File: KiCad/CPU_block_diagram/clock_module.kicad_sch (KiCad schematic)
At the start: 17 parts, among them SW1 SW_Push, U1 LM555xN, U2 LM555xN, U3 LM555xN

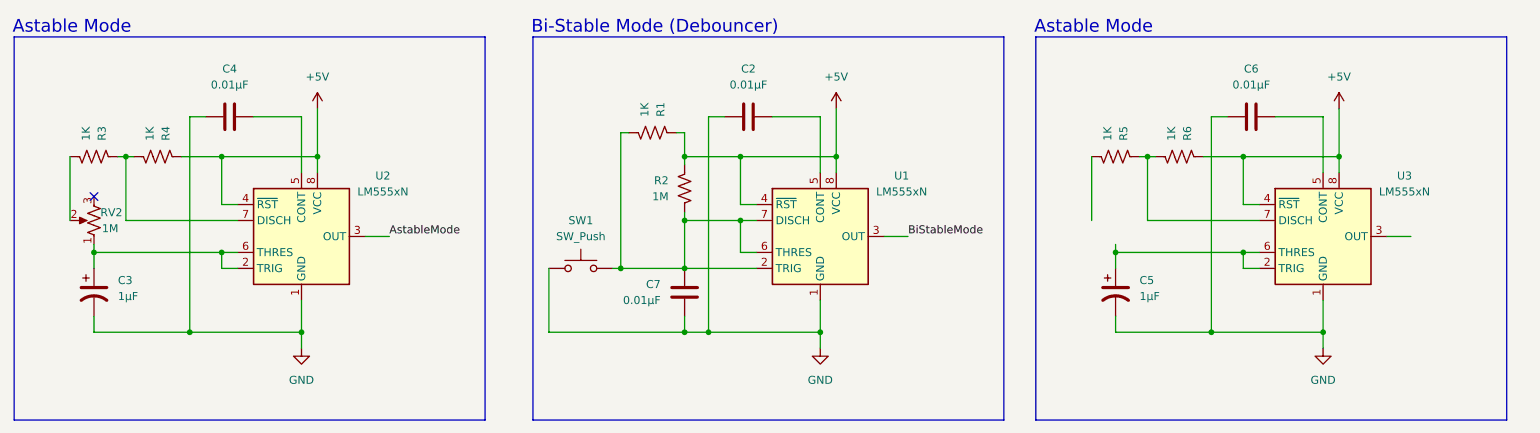
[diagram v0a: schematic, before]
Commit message: vault backup: 2025-12-29 10:56:26
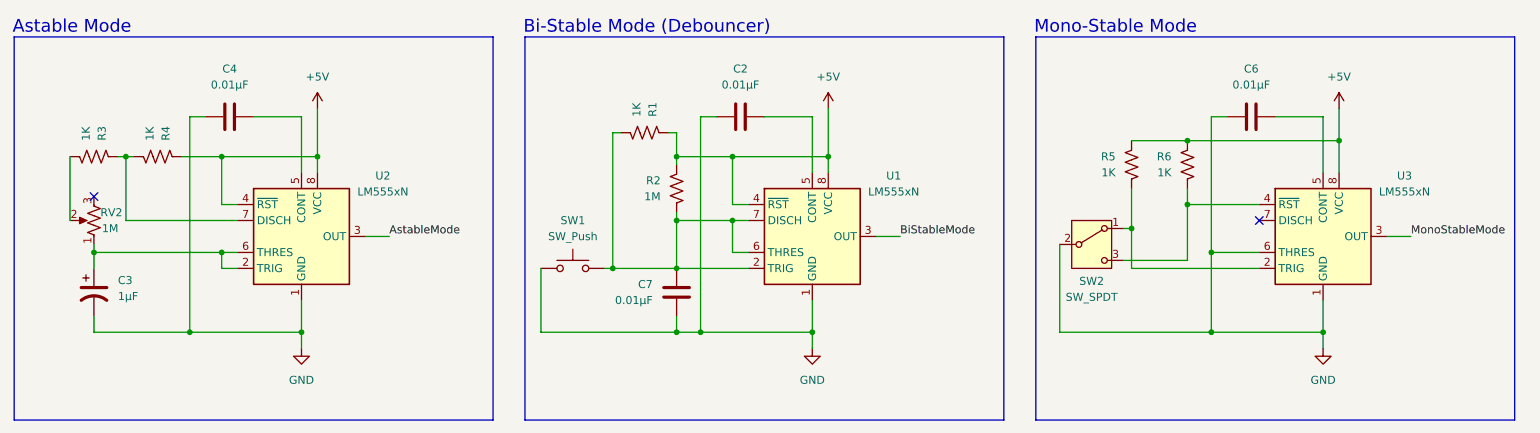
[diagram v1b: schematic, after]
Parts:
- removed C5: 1µF, symbol Device:C_Polarized_US
- added SW2: SW_SPDT, symbol Switch:SW_SPDT
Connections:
- net +5V: now also R5.1; no longer U3.4 (~{RST})
- net GND: now also U3.6 (THRES), SW2.2 (B)
- net at U3.2 (TRIG): now also R5.2, SW2.1 (A); no longer U3.6 (THRES)
- net MonoStableMode: now reaches U3.3 (OUT)
- new net: R6.2, SW2.3 (C), U3.4 (~{RST})
- now unconnected: U3.7 (DISCH)
- no-connect marks 1 -> 2
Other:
- note added: "Mono-Stable Mode"
- moved on the sheet: C2, C7, R1, R2, R5, R6, SW1, U1
